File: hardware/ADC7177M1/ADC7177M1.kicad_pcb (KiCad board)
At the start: 2 copper layers, 132 parts, among them J3 Conn_02x08_Odd_Even, J4 Conn_02x08_Odd_Even, U1 ADG1419BRMZ, U10 ADP7182ACPZN, U11 ADA4522-2ARMZ, U12 AD8066ARMZ, U13 AD7177-2BRUZ, U14 ADR1399KEZ, U15 LT1012S8, U16 ADA4522-1ARMZ, U17 AD8065ART, U2 ADG1419BRMZ, U3 OPA2189IDGK, U4 OPA2388IDGKx, U5 AD8066ARMZ, U6 ADG1408YRUZ, U7 ADG1408YRUZ, U8 ADP7118ACPZN, U9 ADP7118ACPZN, Y1 ECS-2520MV-160-BL-TR

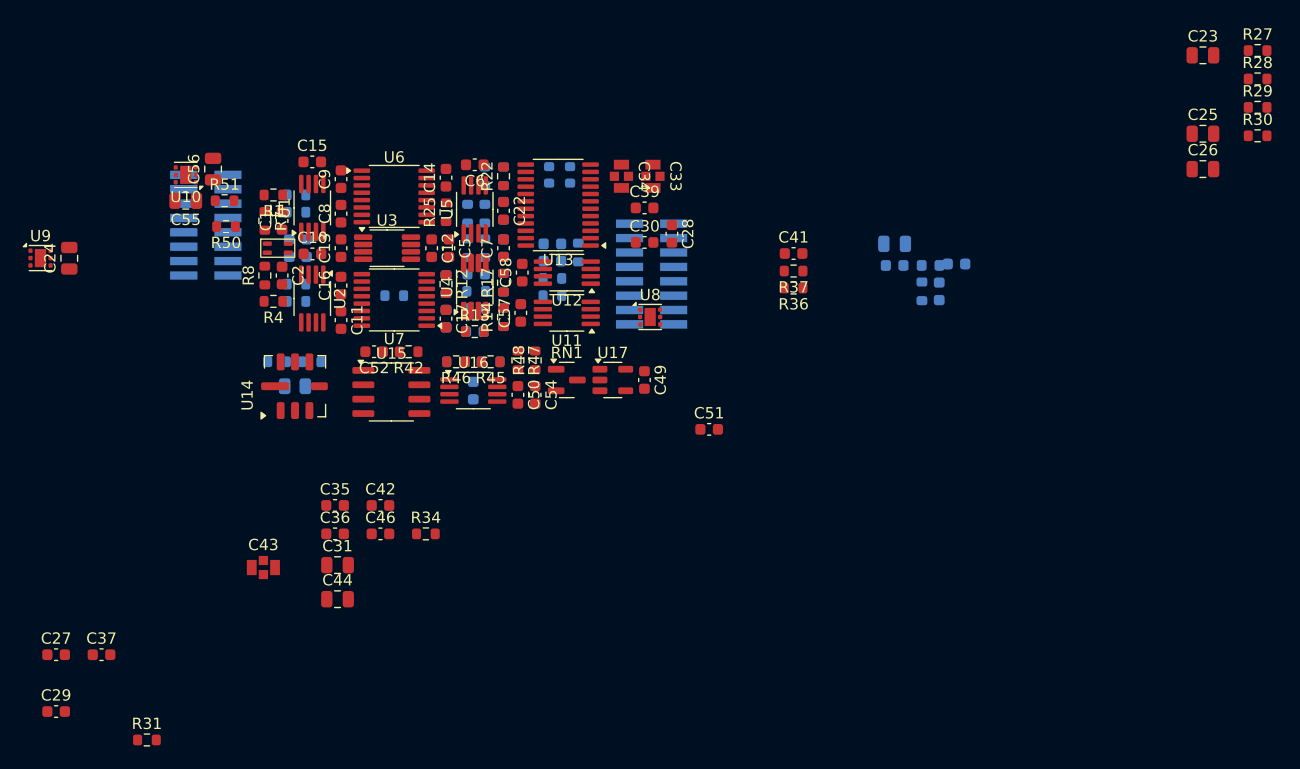
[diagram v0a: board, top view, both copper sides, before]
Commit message: Schematic and PCB
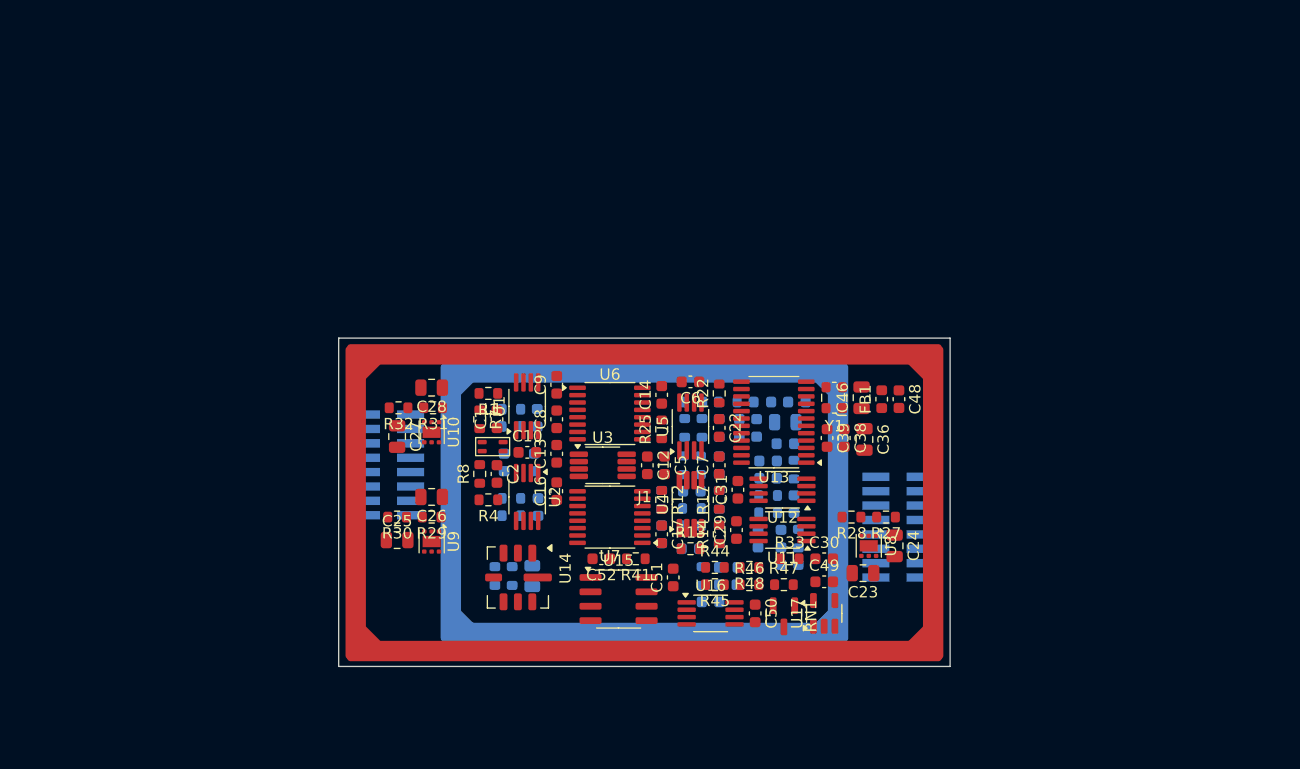
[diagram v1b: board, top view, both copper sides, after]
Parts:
- removed the C33 at (150.4, 64.0)
- removed the C34 at (147.6, 64.0)
- removed the C42 at (126.3, 93.1)
- removed the C43 at (116.0, 98.6)
- removed the R36 at (162.8, 73.9)
- removed the R37 at (162.8, 72.4)
- removed the R38 at (174.1, 74.2)
- added J1: 3670513, ADC7177M1:3670513, F.Cu at (149.6, 92.8)
- added J2: 3670345, ADC7177M1:3670345, B.Cu at (149.6, 92.8)
- C11, C15, C44, C54: moved to B.Cu
- C32: renamed from C28; moved to B.Cu
- C33: renamed from C29; moved to B.Cu
- C34: renamed from C30; moved to B.Cu
- C37: renamed from C35; moved to B.Cu
- C41: renamed from C39; moved to B.Cu
- C43: renamed from C41; moved to B.Cu
- C45: renamed from C46; moved to B.Cu
- C46: renamed from C45; moved to F.Cu
- C48, FB1, Y1: moved to F.Cu
- R36: renamed from R34; moved to B.Cu
- R48: renamed from R49; moved to F.Cu
- moved R30 83.1 mm to (127.8, 94.1), turned to 180 degrees
- moved R29 81.4 mm to (130.8, 94.1), turned to 180 degrees
- moved C26 74.0 mm to (130.8, 92.3), turned to 180 degrees
- moved C30 68.4 mm to (165.5, 97.8)
- moved C39 66.9 mm to (165.7, 87.1), turned to -90 degrees
- moved C33 65.8 mm to (161.7, 96.0), turned to -90 degrees
- moved R33 59.0 mm to (162.4, 97.8)
- moved C23 54.7 mm to (168.9, 99.1), turned to 180 degrees
- moved R28 52.8 mm to (167.9, 94.1), turned to 180 degrees
- moved R27 52.7 mm to (170.9, 94.1), turned to 180 degrees
- moved C36 47.8 mm to (169.0, 87.2), turned to -90 degrees
- moved C38 45.8 mm to (167.3, 87.1), turned to -90 degrees
- moved C24 45.5 mm to (171.7, 96.6), turned to -90 degrees
- moved U9 42.7 mm to (130.8, 96.3), turned to -90 degrees
- moved C44 42.5 mm to (162.1, 85.7)
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- renumbered C25 to C24, C24 to C25, C55 to C27, C56 to C28, C57 to C29, C27 to C30, C58 to C31, C32 to C35, C31 to C36, C36 to C38, C37 to C39, C38 to C40, C40 to C42, R50 to R31, R51 to R32, R31 to R33, R32 to R34, R33 to R35, R35 to R37, R39 to R38, R40 to R39, R41 to R40, R42 to R41, R43 to R42, R44 to R43, R45 to R44, R46 to R45, R47 to R46, R48 to R47
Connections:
- C38 pad 1: Net-(U13-AVDD1) -> +5VA
- C39 pad 1: Net-(U13-AVDD2) -> +5VA
- U13 pad 16: Net-(U13-IOVDD) -> +3.3V
- U13 pad 7: Net-(U13-AVDD1) -> +5VA
- U13 pad 8: Net-(U13-AVDD2) -> +5VA
- Y1 pad 1: Net-(Y1-Tri-State) -> unconnected-(Y1-Tri-State-Pad1)
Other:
- board outline added: 54 x 29 mm
